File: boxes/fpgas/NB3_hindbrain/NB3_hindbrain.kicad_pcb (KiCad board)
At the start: 2 copper layers, 8 parts, among them IC1 NOR_Flash_W25Q32JVSSIQ, IC2 FPGA_ICE40UP5K-SG48I, J1 MicroUSB_10103594-0001LF, U1 USBtoSPI_FT4232HL, U2 EEPROM_93LC56BT-I-OT, Y1 Osc_12MHz_ECS-2520MV-120-BN-TR

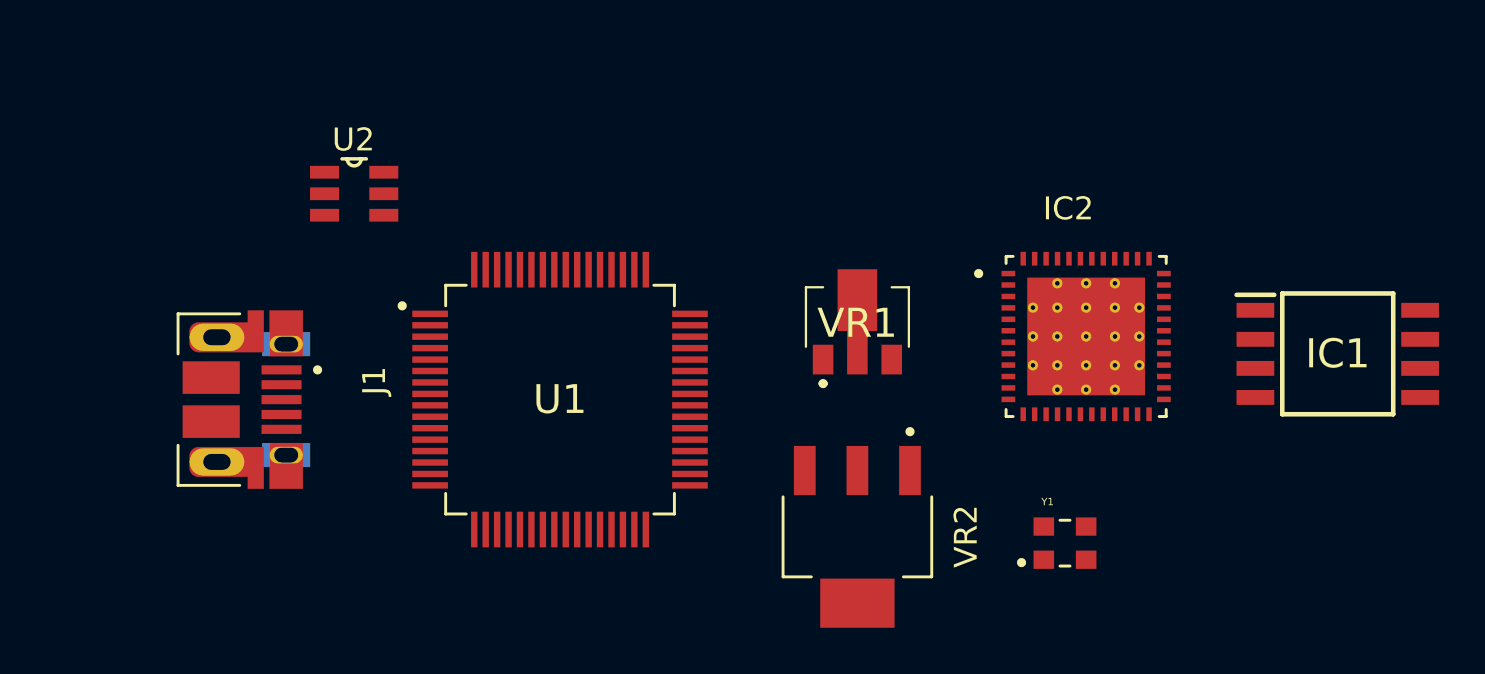
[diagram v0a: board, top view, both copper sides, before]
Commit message: Tweaks to NB3_hindbrain
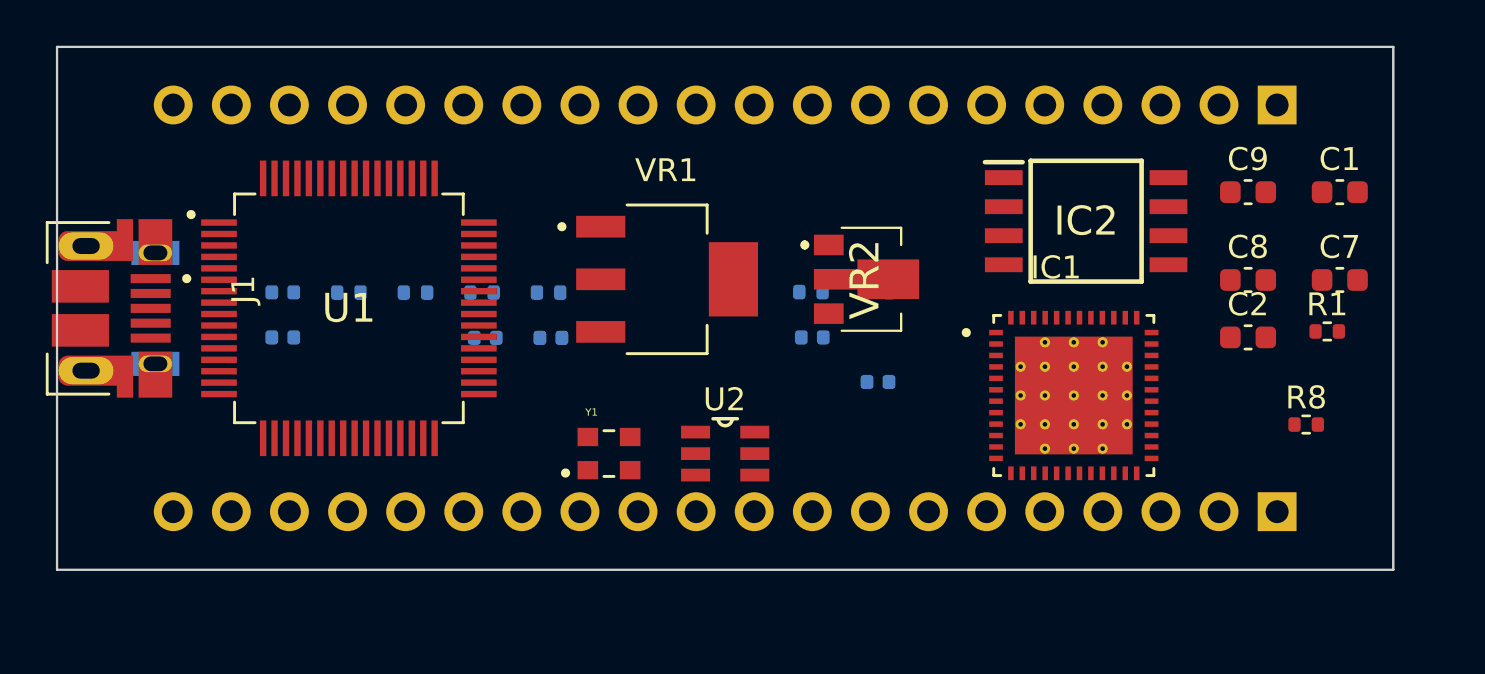
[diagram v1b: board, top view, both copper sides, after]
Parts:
- added C1: 10uF, Capacitor_SMD:C_0603_1608Metric, F.Cu at (136.1, 74.9)
- added C10: 100nF, Capacitor_SMD:C_0402_1005Metric, B.Cu at (89.9, 79.3)
- added C11: 100nF, Capacitor_SMD:C_0402_1005Metric, B.Cu at (113.0, 81.3)
- added C2: 10uF, Capacitor_SMD:C_0603_1608Metric, F.Cu at (132.1, 81.3)
- added C3: 100nF, Capacitor_SMD:C_0402_1005Metric, B.Cu at (115.9, 83.2)
- added C4: 100nF, Capacitor_SMD:C_0402_1005Metric, B.Cu at (101.6, 81.3)
- added C5: 100nF, Capacitor_SMD:C_0402_1005Metric, B.Cu at (89.9, 81.3)
- added C6: 100nF, Capacitor_SMD:C_0402_1005Metric, B.Cu at (98.7, 81.3)
- added C7: 3.3uF, Capacitor_SMD:C_0603_1608Metric, F.Cu at (136.1, 78.8)
- added C8: 10uF, Capacitor_SMD:C_0603_1608Metric, F.Cu at (132.1, 78.8)
- added C9: 10uF, Capacitor_SMD:C_0603_1608Metric, F.Cu at (132.1, 74.9)
- added J2: Conn_01x20_Male, Connector_PinHeader_2.54mm:PinHeader_1x20_P2.54mm_Vertical, B.Cu at (133.3, 71.1)
- added J3: Conn_01x20_Male, Connector_PinHeader_2.54mm:PinHeader_1x20_P2.54mm_Vertical, B.Cu at (133.3, 88.9)
- added R1: 10k, Resistor_SMD:R_0402_1005Metric, F.Cu at (135.5, 81.0)
- added R2: 10k, Resistor_SMD:R_0402_1005Metric, B.Cu at (98.6, 79.3)
- added R3: 2.2k, Resistor_SMD:R_0402_1005Metric, B.Cu at (92.8, 79.3)
- added R4: 4.7k, Resistor_SMD:R_0402_1005Metric, B.Cu at (115.9, 79.3)
- added R5: 10k, Resistor_SMD:R_0402_1005Metric, B.Cu at (95.7, 79.3)
- added R6: 10k, Resistor_SMD:R_0402_1005Metric, B.Cu at (113.0, 79.3)
- added R7: 1k, Resistor_SMD:R_0402_1005Metric, B.Cu at (101.5, 79.3)
- added R8: 12k, Resistor_SMD:R_0402_1005Metric, F.Cu at (134.6, 85.1)
- IC1: value NOR_Flash_W25Q32JVSSIQ -> FPGA_ICE40UP5K-SG48I; footprint NB3_hindbrain:NOR_Flash_W25Q32JVSSIQ -> NB3_hindbrain:FPGA_ICE40UP5K-SG48I
- IC2: value FPGA_ICE40UP5K-SG48I -> NOR_Flash_W25Q32JVSSIQ; footprint NB3_hindbrain:FPGA_ICE40UP5K-SG48I -> NB3_hindbrain:NOR_Flash_W25Q32JVSSIQ
- VR1: value LDO_1v2_AP7217D-12YG-13 -> LDO_3v3_LM1117IMPX-3.3; footprint NB3_hindbrain:LDO_1v2_AP7217D-12YG-13 -> NB3_hindbrain:LDO_3v3_LM1117IMPX-3.3
- VR2: value LDO_3v3_LM1117IMPX-3.3 -> LDO_1v2_AP7217D-12YG-13; footprint NB3_hindbrain:LDO_3v3_LM1117IMPX-3.3 -> NB3_hindbrain:LDO_1v2_AP7217D-12YG-13
- moved Y1 20.3 mm to (104.1, 86.4)
- moved U2 19.8 mm to (109.2, 86.4)
- moved IC1 11.7 mm to (124.5, 83.8)
- moved VR2 11.3 mm to (115.0, 78.7)
- moved U1 10.1 mm to (92.8, 80.0)
- moved VR1 8.62 mm to (106.7, 78.7)
- moved J1 6.97 mm to (81.3, 80.0)
- moved IC2 5.04 mm to (125.0, 76.2)
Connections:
- net /EEDATA renamed /EEDATA_I
- IC2 pad 2: unconnected-(IC2-Pad2) -> /FPGA_SI
- IC2 pad 4: unconnected-(IC2-Pad4) -> GND
- IC2 pad 5: unconnected-(IC2-Pad5) -> /FPGA_SO
- IC2 pad 6: unconnected-(IC2-Pad6) -> /FPGA_SCK
- IC2 pad 8: unconnected-(IC2-Pad8) -> +3V3
- J1 pad 1: unconnected-(J1-Pad1) -> Net-(J1-Pad1)
- U1 pad 12: unconnected-(U1-Pad12) -> +1V8
- U1 pad 13: unconnected-(U1-Pad13) -> GND
- U1 pad 14: unconnected-(U1-Pad14) -> Net-(R7-Pad2)
- U1 pad 20: unconnected-(U1-Pad20) -> +3V3
- U1 pad 31: unconnected-(U1-Pad31) -> +3V3
- U1 pad 37: unconnected-(U1-Pad37) -> +1V8
- U1 pad 42: unconnected-(U1-Pad42) -> +3V3
- U1 pad 49: unconnected-(U1-Pad49) -> +1V8
- U1 pad 50: unconnected-(U1-Pad50) -> +3V3
- U1 pad 56: unconnected-(U1-Pad56) -> +3V3
- U1 pad 6: unconnected-(U1-Pad6) -> Net-(R8-Pad1)
- U1 pad 64: unconnected-(U1-Pad64) -> +1V8
- U2 pad 1: unconnected-(U2-Pad1) -> /EEDATA_O
- U2 pad 6: unconnected-(U2-Pad6) -> +3V3
- VR1 pad 1: unconnected-(VR1-Pad1) -> GND
- VR1 pad 2: unconnected-(VR1-Pad2) -> +3V3
- VR1 pad 3: unconnected-(VR1-Pad3) -> +5V
- VR1 pad 4: unconnected-(VR1-Pad4) -> +3V3
- VR2 pad 1: unconnected-(VR2-Pad1) -> GND
- VR2 pad 2: unconnected-(VR2-Pad2) -> +5V
- VR2 pad 3: unconnected-(VR2-Pad3) -> +1V2
- VR2 pad 4: unconnected-(VR2-Pad4) -> +5V
- Y1 pad 2: unconnected-(Y1-Pad2) -> GND
- Y1 pad 4: unconnected-(Y1-Pad4) -> +3V3
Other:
- board outline added: 58.4 x 22.9 mm
